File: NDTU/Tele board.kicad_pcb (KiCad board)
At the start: 2 copper layers, 9 parts, among them U1 STM32H573VITx, U10 TLV75533PDRV, U12 AMS1117, U2 BMP280, U3 MS5611-01BA, U4 BMI088, U7 TPS565208, U8 TPS62162DSG

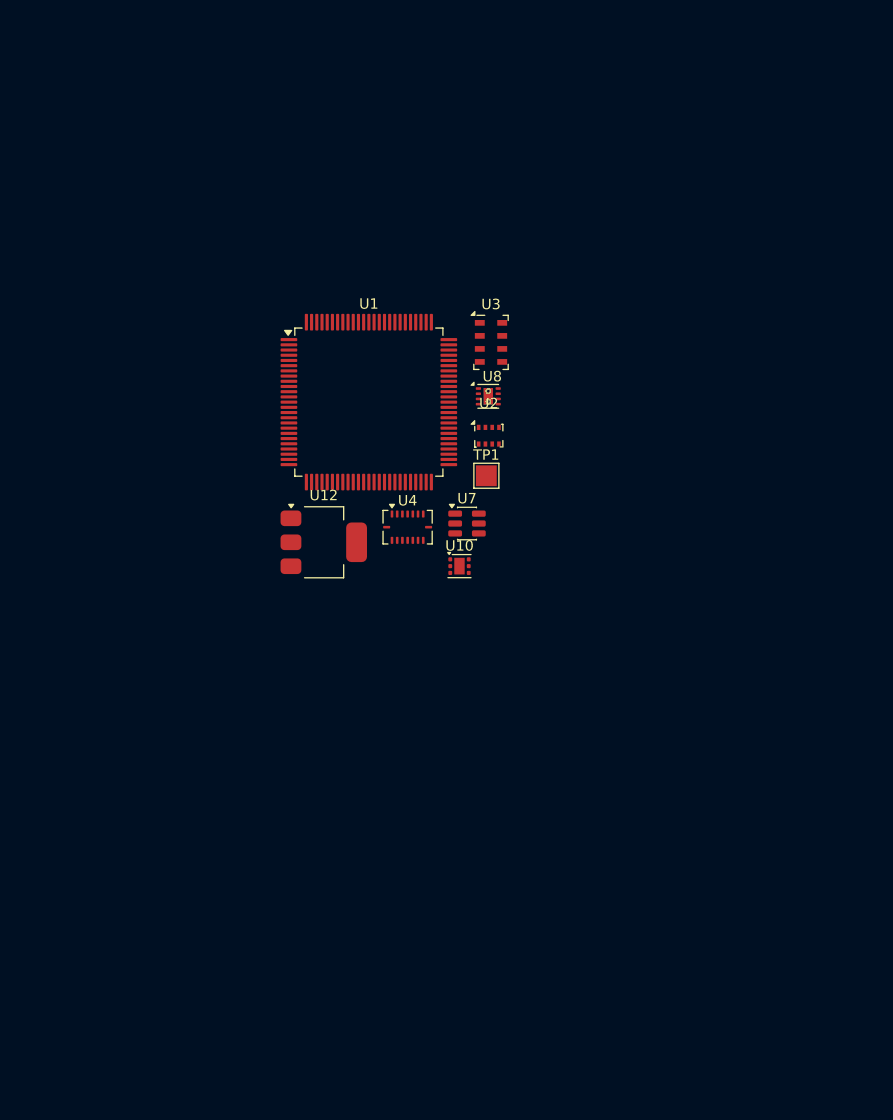
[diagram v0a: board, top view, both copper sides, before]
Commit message: Add files via upload
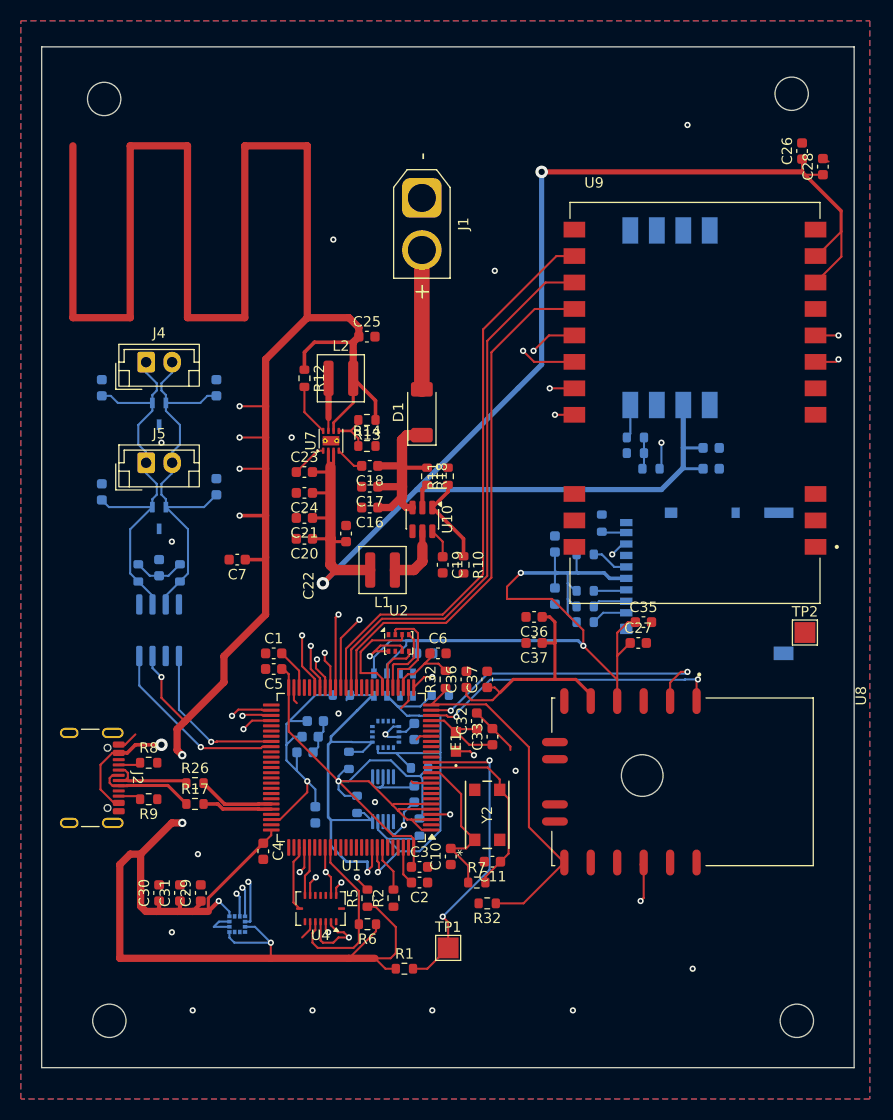
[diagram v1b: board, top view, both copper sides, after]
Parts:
- removed U12: AMS1117, Package_TO_SOT_SMD:SOT-223-3_TabPin2
- added ?: , , F.Cu at (112.5, 144.0)
- added ?: , , F.Cu at (178.5, 144.0)
- added ?: , , F.Cu at (112.0, 55.5)
- added ?: , , F.Cu at (178.0, 55.0)
- added C1: 2.2uF, Capacitor_SMD:C_0603_1608Metric, F.Cu at (128.3, 108.7)
- added C10: 22pF, Capacitor_SMD:C_0603_1608Metric, F.Cu at (145.3, 128.2)
- added C11: 22pF, Capacitor_SMD:C_0603_1608Metric, F.Cu at (149.3, 128.7)
- added C12: 1uF, Capacitor_SMD:C_0603_1608Metric, B.Cu at (132.3, 115.2)
- added C13: 100nF, Capacitor_SMD:C_0603_1608Metric, B.Cu at (131.8, 116.7)
- added C14: 100nF, Capacitor_SMD:C_0603_1608Metric, B.Cu at (131.3, 118.2)
- added C15: 10uF, Capacitor_SMD:C_0603_1608Metric, B.Cu at (141.8, 116.2)
- added C16: 10uF, Capacitor_SMD:C_0603_1608Metric, F.Cu at (137.5, 94.7)
- added C17: 10uF, Capacitor_SMD:C_0603_1608Metric, F.Cu at (137.5, 92.7)
- added C18: 100nF, Capacitor_SMD:C_0603_1608Metric, F.Cu at (137.5, 90.7)
- added C19: 100nF, Capacitor_SMD:C_0603_1608Metric, F.Cu at (144.5, 100.2)
- added C2: 2.2uF, Capacitor_SMD:C_0603_1608Metric, F.Cu at (142.3, 130.7)
- added C20: 22uF, Capacitor_SMD:C_0603_1608Metric, F.Cu at (131.2, 97.7)
- added C21: 22uF, Capacitor_SMD:C_0603_1608Metric, F.Cu at (131.2, 95.7)
- added C22: 100nF, Capacitor_SMD:C_0603_1608Metric, F.Cu at (135.2, 97.2)
- added C23: 10uF, Capacitor_SMD:C_0603_1608Metric, F.Cu at (131.2, 91.3)
- added C24: 100nF, Capacitor_SMD:C_0603_1608Metric, F.Cu at (131.2, 93.3)
- added C25: 22uF, Capacitor_SMD:C_0603_1608Metric, F.Cu at (137.2, 78.3)
- added C26: 100nF, Capacitor_SMD:C_0603_1608Metric, F.Cu at (179.0, 60.5)
- added C27: 10uF, Capacitor_SMD:C_0603_1608Metric, F.Cu at (163.3, 107.7)
- added C28: 10uF, Capacitor_SMD:C_0603_1608Metric, F.Cu at (181.0, 62.0)
- added C29: 100nF, Capacitor_SMD:C_0603_1608Metric, F.Cu at (121.3, 131.7)
- added C3: 100nF, Capacitor_SMD:C_0603_1608Metric, F.Cu at (142.3, 129.2)
- added C30: 100nF, Capacitor_SMD:C_0603_1608Metric, F.Cu at (117.3, 131.7)
- added C31: 1uF, Capacitor_SMD:C_0603_1608Metric, F.Cu at (119.3, 131.7)
- added C32: 100nF, Capacitor_SMD:C_0603_1608Metric, F.Cu at (147.8, 115.2)
- added C33: 1uF, Capacitor_SMD:C_0603_1608Metric, F.Cu at (149.3, 116.7)
- added C34: 10nF, Capacitor_SMD:C_0603_1608Metric, B.Cu at (170.3, 91.0)
- added C35: 100uF, Capacitor_SMD:C_0603_1608Metric, F.Cu at (163.8, 105.7)
- added C36: 100nF, Capacitor_SMD:C_0603_1608Metric, F.Cu at (153.3, 105.2)
- added C36: 100nF, Capacitor_SMD:C_0603_1608Metric, F.Cu at (146.8, 111.2)
- added C37: 4.7uF, Capacitor_SMD:C_0603_1608Metric, F.Cu at (153.3, 107.7)
- added C37: 4.7uF, Capacitor_SMD:C_0603_1608Metric, F.Cu at (148.8, 111.2)
- added C38: 100nF, Capacitor_SMD:C_0603_1608Metric, B.Cu at (155.3, 98.2)
- added C39: 10uF, Capacitor_SMD:C_0603_1608Metric, B.Cu at (155.3, 103.2)
- added C4: 100nF, Capacitor_SMD:C_0603_1608Metric, F.Cu at (127.3, 127.7)
- added C40: 47pF, Capacitor_SMD:C_0603_1608Metric, B.Cu at (122.8, 92.7)
- added C41: 47pF, Capacitor_SMD:C_0603_1608Metric, B.Cu at (111.8, 93.2)
- added C42: 4.7nF, Capacitor_SMD:C_0603_1608Metric, B.Cu at (117.3, 100.5)
- added C43: 47pF, Capacitor_SMD:C_0603_1608Metric, B.Cu at (122.8, 83.2)
- added C44: 47pF, Capacitor_SMD:C_0603_1608Metric, B.Cu at (111.8, 83.2)
- added C45: 1uF, Capacitor_SMD:C_0603_1608Metric, B.Cu at (170.3, 89.0)
- added C46: 100nF, Capacitor_SMD:C_0603_1608Metric, B.Cu at (141.8, 122.2)
- added C5: 100nF, Capacitor_SMD:C_0603_1608Metric, F.Cu at (128.3, 110.2)
- added C6: 100nF, Capacitor_SMD:C_0603_1608Metric, F.Cu at (144.1, 108.7)
- added C7: 1uF, Capacitor_SMD:C_0603_1608Metric, F.Cu at (124.8, 99.7)
- added C8: 100nF, Capacitor_SMD:C_0603_1608Metric, B.Cu at (142.8, 108.7)
- added C9: 100nF, Capacitor_SMD:C_0603_1608Metric, B.Cu at (132.3, 124.2)
- added CR3: ESDCAN02-2BWY, ESDCAN02-2BWY:SOT323-3L_STM, B.Cu at (117.3, 85.7)
- added CR3: ESDCAN02-2BWY, ESDCAN02-2BWY:SOT323-3L_STM, B.Cu at (117.3, 95.7)
- added D1: D_Schottky, Diode_SMD:D_SOD-128, F.Cu at (142.5, 85.6)
- added E1: LI0603G121R-10, NewLib:IND_LI0603G121R-10_LRD-M, F.Cu at (145.8, 117.2)
- added IC1: MPXV5100DP, NewLib:MPXV5100DP, B.Cu at (169.5, 76.5)
- added J1: Conn_01x02, Connector_AMASS:AMASS_XT30U-M_1x02_P5.0mm_Vertical, F.Cu at (142.5, 65.0)
- added J2: USB_C_Receptacle_USB2.0_16P, Connector_USB:USB_C_Receptacle_GCT_USB4105-xx-A_16P_TopMnt_Horizontal, F.Cu at (109.7, 120.7)
- added J3: Micro_SD_Card, Connector_Card:microSD_HC_Hirose_DM3AT-SF-PEJM5, B.Cu at (169.8, 102.0)
- added J4: Conn_01x02_Pin, Connector_JST:JST_EH_B2B-EH-A_1x02_P2.50mm_Vertical, F.Cu at (116.0, 80.8)
- added J5: Conn_01x02_Pin, Connector_JST:JST_EH_B2B-EH-A_1x02_P2.50mm_Vertical, F.Cu at (116.0, 90.4)
- added L1: 4.7uH, Inductor_SMD:L_Coilcraft_XAL4020-XXX, F.Cu at (138.7, 100.7)
- added L2: 2.2uH, Inductor_SMD:L_Coilcraft_XAL4020-XXX, F.Cu at (134.7, 82.3)
- added R1: 10k, Resistor_SMD:R_0603_1608Metric, F.Cu at (140.8, 139.0)
- added R10: 56.2k, Resistor_SMD:R_0603_1608Metric, F.Cu at (146.5, 100.2)
- added R11: 10k, Resistor_SMD:R_0603_1608Metric, F.Cu at (145.0, 91.7)
- added R12: 100k, Resistor_SMD:R_0603_1608Metric, F.Cu at (131.2, 82.3)
- added R13: 470k, Resistor_SMD:R_0603_1608Metric, F.Cu at (137.2, 86.3)
- added R14: 150k, Resistor_SMD:R_0603_1608Metric, F.Cu at (137.2, 88.8)
- added R15: 10k, Resistor_SMD:R_0603_1608Metric, B.Cu at (135.5, 119.0)
- added R16: 10k, Resistor_SMD:R_0603_1608Metric, B.Cu at (142.3, 119.7)
- added R17: 27, Resistor_SMD:R_0603_1608Metric, F.Cu at (120.7, 123.2)
- added R18: 10k, Resistor_SMD:R_0603_1608Metric, F.Cu at (143.0, 91.7)
- added R19: 10k, Resistor_SMD:R_0603_1608Metric, B.Cu at (158.2, 105.7)
- added R2: 10k, Resistor_SMD:R_0603_1608Metric, F.Cu at (139.8, 132.2)
- added R20: 10k, Resistor_SMD:R_0603_1608Metric, B.Cu at (158.2, 104.2)
- added R21: 10k, Resistor_SMD:R_0603_1608Metric, B.Cu at (158.2, 102.7)
- added R22: 10k, Resistor_SMD:R_0603_1608Metric, B.Cu at (158.2, 99.2)
- added R23: 10k, Resistor_SMD:R_0603_1608Metric, B.Cu at (159.8, 96.2)
- added R24: 60, Resistor_SMD:R_0603_1608Metric, B.Cu at (119.3, 101.0)
- added R25: 60, Resistor_SMD:R_0603_1608Metric, B.Cu at (115.3, 101.0)
- added R26: 27, Resistor_SMD:R_0603_1608Metric, F.Cu at (120.7, 121.2)
- added R27: 100, Resistor_SMD:R_0603_1608Metric, B.Cu at (163.0, 88.0)
- added R28: 4.7k, Resistor_SMD:R_0603_1608Metric, B.Cu at (136.3, 123.2)
- added R29: 4.7k, Resistor_SMD:R_0603_1608Metric, B.Cu at (144.3, 112.7)
- added R3: 4.7k, Resistor_SMD:R_0603_1608Metric, B.Cu at (142.3, 125.4)
- added R30: 20k, Resistor_SMD:R_0603_1608Metric, B.Cu at (163.0, 89.5)
- added R31: 10k, Resistor_SMD:R_0603_1608Metric, B.Cu at (164.5, 91.0)
- added R32: 10k, Resistor_SMD:R_0603_1608Metric, F.Cu at (148.8, 132.7)
- added R32: 10k, Resistor_SMD:R_0603_1608Metric, F.Cu at (144.8, 111.2)
- added R4: 4.7k, Resistor_SMD:R_0603_1608Metric, B.Cu at (134.8, 112.7)
- added R5: 10k, Resistor_SMD:R_0603_1608Metric, F.Cu at (137.3, 132.2)
- added R6: 10k, Resistor_SMD:R_0603_1608Metric, F.Cu at (137.3, 134.7)
- added R7: 1M, Resistor_SMD:R_0603_1608Metric, F.Cu at (147.8, 130.7)
- added R8: 5.1k, Resistor_SMD:R_0603_1608Metric, F.Cu at (116.3, 119.2)
- added R9: 5.1k, Resistor_SMD:R_0603_1608Metric, F.Cu at (116.3, 122.7)
- added TP2: TestPoint, TestPoint:TestPoint_Pad_2.0x2.0mm, F.Cu at (179.3, 106.7)
- added U13: TCAN332, Package_SO:SOIC-8_3.9x4.9mm_P1.27mm, B.Cu at (117.3, 106.5)
- added U14: ADS1115IDGS, Package_SO:TSSOP-10_3x3mm_P0.5mm, B.Cu at (138.8, 122.7)
- added U5: MMC5983MA, NewLib:PQFN50P300X300X100-16N, B.Cu at (139.0, 116.5)
- added U6: KX134-1211, NewLib:LGA12_2X2X0P9_ROM-M, B.Cu at (124.8, 134.7)
- added U9: E22-900M30S, NewLib:XCVR_E22-900M30S, F.Cu at (168.7, 84.7)
- added Y2: ABMM2-8MHz, NewLib:CRYSTAL_ABMM2_ABR, F.Cu at (148.8, 124.2)
- U10: value TLV75533PDRV -> AP63200WU; footprint Package_SON:WSON-6-1EP_2x2mm_P0.65mm_EP1x1.6mm -> Package_TO_SOT_SMD:TSOT-23-6
- U3: moved to B.Cu
- U7: value TPS565208 -> TPS62162DSG; footprint Package_TO_SOT_SMD:SOT-23-6 -> Package_SON:Texas_DSG0008A_WSON-8-1EP_2x2mm_P0.5mm_EP0.9x1.6mm_ThermalVias
- U8: value TPS62162DSG -> L89; footprint Package_SON:WSON-8-1EP_2x2mm_P0.5mm_EP0.9x1.6mm_ThermalVias -> NewLib:XCVR_L89
- moved TP1 45.5 mm to (145.0, 137.0)
- moved U8 41.4 mm to (167.5, 121.1), turned to -90 degrees
- moved U4 37.6 mm to (132.8, 133.2), turned to 180 degrees
- moved U1 35.1 mm to (135.7, 119.7), turned to 180 degrees
- moved U3 34.2 mm to (139.8, 111.7), turned to -90 degrees
- moved U2 21.7 mm to (140.3, 107.7)
- moved U7 15.3 mm to (133.8, 88.3), turned to 90 degrees
- moved U10 5.73 mm to (142.6, 95.9), turned to -90 degrees
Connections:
- U1 pad 1: unconnected-(U1-PE2-Pad1) -> +3V3
- U1 pad 15: unconnected-(U1-PC0-Pad15) -> /PC0
- U1 pad 16: unconnected-(U1-PC1-Pad16) -> /PC1
- U1 pad 17: unconnected-(U1-PC2-Pad17) -> /PC2
- U1 pad 18: unconnected-(U1-PC3-Pad18) -> /PC3
- U1 pad 2: unconnected-(U1-PE3-Pad2) -> /PE3
- U1 pad 22: +3V3 -> Net-(U1-VDDA)
- U1 pad 23: unconnected-(U1-PA0-Pad23) -> GNSS_RX
- U1 pad 24: unconnected-(U1-PA1-Pad24) -> GNSS_TX
- U1 pad 25: unconnected-(U1-PA2-Pad25) -> GNSS_WU
- U1 pad 26: unconnected-(U1-PA3-Pad26) -> /PA3
- U1 pad 3: unconnected-(U1-PE4-Pad3) -> +3V3
- U1 pad 33: unconnected-(U1-PC4-Pad33) -> /PC4
- U1 pad 34: unconnected-(U1-PC5-Pad34) -> /PC5
- U1 pad 35: unconnected-(U1-PB0-Pad35) -> /PB0
- U1 pad 36: unconnected-(U1-PB1-Pad36) -> /PB1
- U1 pad 37: unconnected-(U1-PB2-Pad37) -> /PB2
- U1 pad 38: unconnected-(U1-PE7-Pad38) -> /PE7
- U1 pad 39: unconnected-(U1-PE8-Pad39) -> /PE8
- U1 pad 4: unconnected-(U1-PE5-Pad4) -> /SD_MISO
- U1 pad 40: unconnected-(U1-PE9-Pad40) -> /PE9
- U1 pad 41: unconnected-(U1-PE10-Pad41) -> /PE10
- U1 pad 46: unconnected-(U1-PE15-Pad46) -> /PE15
- U1 pad 47: unconnected-(U1-PB10-Pad47) -> /PB10
- U1 pad 5: unconnected-(U1-PE6-Pad5) -> +3V3
- U1 pad 55: unconnected-(U1-PD8-Pad55) -> /PD8
- U1 pad 56: unconnected-(U1-PD9-Pad56) -> /PD9
- U1 pad 57: unconnected-(U1-PD10-Pad57) -> /PD10
- U1 pad 58: unconnected-(U1-PD11-Pad58) -> CAN_TX
- U1 pad 59: unconnected-(U1-PD12-Pad59) -> CAN_RX
- U1 pad 60: unconnected-(U1-PD13-Pad60) -> /PD13
- U1 pad 61: unconnected-(U1-PD14-Pad61) -> /PD14
- U1 pad 62: unconnected-(U1-PD15-Pad62) -> /PD15
- U1 pad 63: unconnected-(U1-PC6-Pad63) -> /PC6
- U1 pad 64: unconnected-(U1-PC7-Pad64) -> /PC7
- U1 pad 65: unconnected-(U1-PC8-Pad65) -> /PC8
- U1 pad 66: unconnected-(U1-PC9-Pad66) -> /PC9
- U1 pad 67: unconnected-(U1-PA8-Pad67) -> /PA8
- U1 pad 68: unconnected-(U1-PA9-Pad68) -> /PA9
- U1 pad 69: unconnected-(U1-PA10-Pad69) -> /PA10
- U1 pad 7: unconnected-(U1-PC13-Pad7) -> /PC13
- U1 pad 70: /USB_DM -> /USB-
- U1 pad 71: /USB_DP -> /USB+
- U1 pad 72: unconnected-(U1-PA13(JTMS-Pad72) -> /PA13(JTMS
- U1 pad 76: unconnected-(U1-PA14(JTCK-Pad76) -> /PA14(JTCK
- U1 pad 77: unconnected-(U1-PA15(JTDI)-Pad77) -> /PA15(JTDI)
- U1 pad 8: unconnected-(U1-PC14-Pad8) -> /PC14
- U1 pad 89: unconnected-(U1-PB3(JTDO-Pad89) -> /PB3(JTDO
- U1 pad 9: unconnected-(U1-PC15-Pad9) -> /PC15
- U1 pad 90: unconnected-(U1-PB4(NJTRST)-Pad90) -> /PB4(NJTRST)
- U1 pad 91: unconnected-(U1-PB5-Pad91) -> /I2C4_SMBA
- U1 pad 92: unconnected-(U1-PB6-Pad92) -> /I2C4_SCL
- U1 pad 93: unconnected-(U1-PB7-Pad93) -> /I2C4_SDA
- U1 pad 97: unconnected-(U1-PE0-Pad97) -> /PE0
- U10 pad 1: +3V3 -> Net-(U10-FB)
- U10 pad 2: unconnected-(U10-NC-Pad2) -> Net-(U10-EN)
- U10 pad 3: GND -> /V_IN
- U10 pad 4: Net-(U10-EN) -> GND
- U10 pad 5: unconnected-(U10-NC-Pad5) -> Net-(U10-SW)
- U3 pad 2: GND -> +3V3
- U3 pad 6: GND -> unconnected-(U3-SDO-Pad6)
- U3 pad 7: /I2C1_SDA -> /I2C4_SDA
- U3 pad 8: /I2C1_SCL -> /I2C4_SCL
- U7 pad 2: Net-(U7-SW) -> +5V
- U7 pad 3: /BAT+ -> +5V
- U7 pad 4: Net-(U7-VFB) -> GND
- U7 pad 6: Net-(U7-VBST) -> +3V3
- U8 pad 1: GND -> GNSS_RX
- U8 pad 2: +5V -> GNSS_TX
- U8 pad 3: +5V -> GND
- U8 pad 4: GND -> +3V3
- U8 pad 6: +3V3 -> unconnected-(U8-1PPS-Pad6)
- U8 pad 7: Net-(U8-SW) -> GNSS_WU
- U8 pad 8: Net-(U8-PG) -> unconnected-(U8-AADET_N-Pad8)
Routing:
- net +3V3: track 0.00 -> 596.1 mm, vias 0 -> 16
- net +5V: track 0.00 -> 191.3 mm, vias 0 -> 3
- net /PE10: track 0.00 -> 68.4 mm, vias 0 -> 2
- net /PE9: track 0.00 -> 66.9 mm, vias 0 -> 2
- net /PE8: track 0.00 -> 55.0 mm
- net Net-(U14-AIN3): track 0.00 -> 55.0 mm, vias 0 -> 2
- net /PE7: track 0.00 -> 52.9 mm
- net /PB2: track 0.00 -> 50.8 mm
- net /PA3: track 0.00 -> 48.2 mm, vias 0 -> 2
- net /I2C4_SDA: track 0.00 -> 47.7 mm, vias 0 -> 1
- net /SPI4_MOSI: track 0.00 -> 47.0 mm, vias 0 -> 2
- net /SPI4_MISO: track 0.00 -> 46.8 mm, vias 0 -> 2
- net GND: track 0.00 -> 45.8 mm, vias 0 -> 18
- net /SPI4_SCK: track 0.00 -> 40.8 mm, vias 0 -> 2
- net /I2C4_SCL: track 0.00 -> 39.4 mm, vias 0 -> 1
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- added copper zone on B.Cu, net GND
- added copper zone on F.Cu, net GND
- added copper zone on In1.Cu, net GND
- added copper zone on In2.Cu, net GND
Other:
- board outline added: 78 x 98 mm
- copper layers 2 -> 4
